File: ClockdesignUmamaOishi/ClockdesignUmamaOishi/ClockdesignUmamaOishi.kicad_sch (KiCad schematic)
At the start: 6 parts

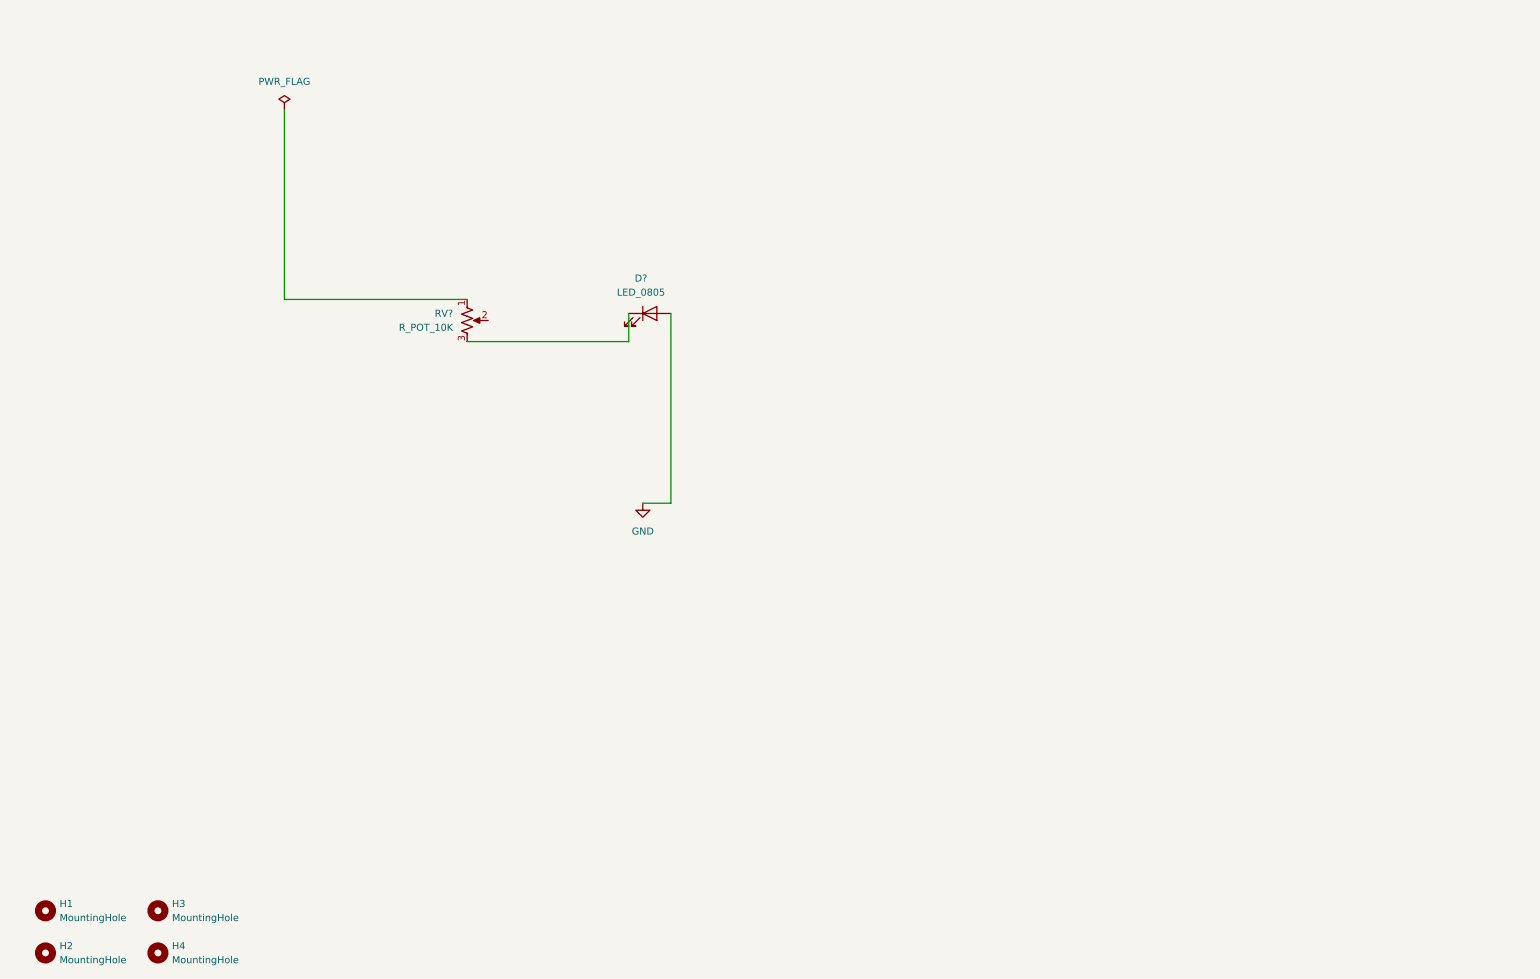
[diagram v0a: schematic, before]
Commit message: Week 2 schematics
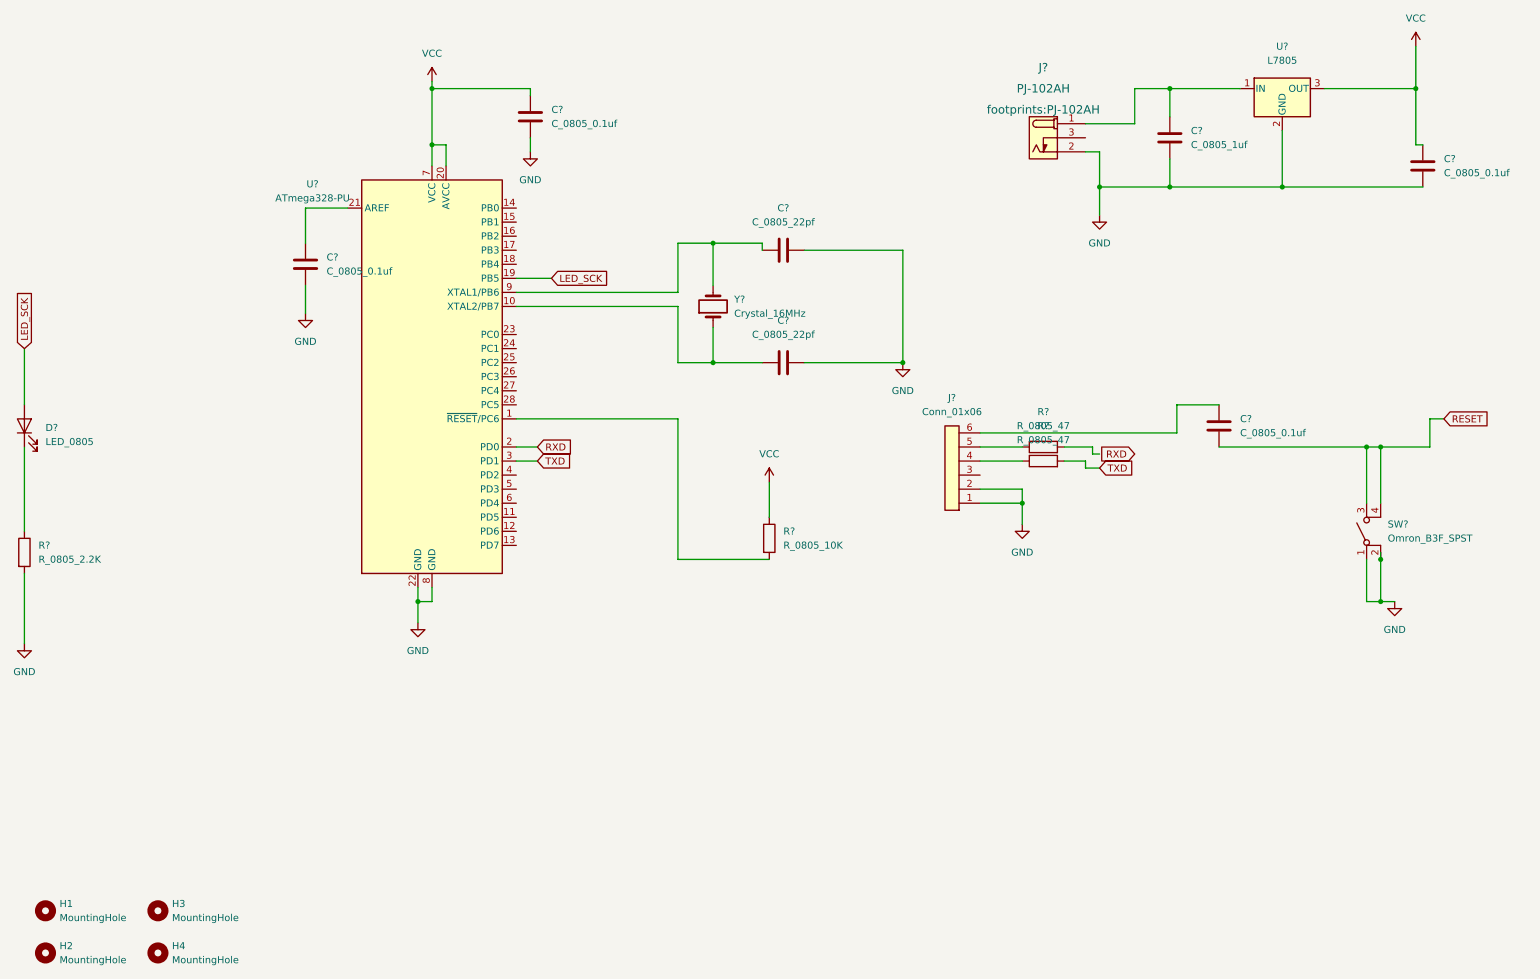
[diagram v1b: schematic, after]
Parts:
- removed D?: LED_0805, footprints:LED_0805_2012Metric, symbol HPS:LED_0805
- removed RV?: R_POT_10K, footprints:Potentiometer_Bourns_3386P_Vertical, symbol HPS:R_POT_10K
- added C? (x4): C_0805_0.1uf, footprints:C_0805_2012Metric, symbol HPS:C_0805_0.1uf
- added C?: C_0805_1uf, footprints:C_0805_2012Metric, symbol HPS:C_0805_1uf
- added C? (x2): C_0805_22pf, footprints:C_0805_2012Metric, symbol HPS:C_0805_22pf
- added D?: LED_0805, footprints:LED_0805_2012Metric, symbol HPS:LED_0805
- added J?: Conn_01x06, footprints:PinHeader_1x06_P2.54mm_Vertical, symbol HPS:Conn_01x06
- added J?: PJ-102AH, footprints:PJ-102AH, symbol HPS:PJ-102AH
- added R?: R_0805_10K, footprints:R_0805_2012Metric, symbol HPS:R_0805_10K
- added R?: R_0805_2.2K, footprints:R_0805_2012Metric, symbol HPS:R_0805_2.2K
- added R? (x2): R_0805_47, footprints:R_0805_2012Metric, symbol HPS:R_0805_47
- added SW?: Omron_B3F_SPST, footprints:SW_SPST_Omron_B3FS-100xP, symbol HPS:Omron_B3F_SPST
- added U?: L7805, symbol HPS:L7805
- added U?: ATmega328-PU, footprints:DIP-28_W7.62mm, symbol HPS:ATmega328-PU
- added Y?: Crystal_16MHz, footprints:Crystal_SMD_HC49-SD, symbol HPS:Crystal_16MHz
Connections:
- net GND: now also C?.2, C?.2, C?.2, C?.2, C?.2, C?.2, J?.1 (Pin_1), J?.2 (OUT), J?.2 (Pin_2), R?.2, SW?.1 (A), SW?.2 (A), U?.2 (GND), U?.22 (GND), U?.8 (GND)
- new net: C?.1, J?.1 (POLE), U?.1 (IN)
- new net: R?.2, U?.1 (~{RESET}/PC6)
- new net: J?.4 (Pin_4), R?.1
- new net: J?.5 (Pin_5), R?.1
- new net: C?.1, J?.6 (Pin_6)
- new net: C?.1, U?.9 (XTAL1/PB6), Y?.2
- new net: D?.1 (K), R?.1
- new net: C?.1, U?.21 (AREF)
- new net: C?.1, U?.10 (XTAL2/PB7), Y?.1
- new net LED_SCK: D?.2 (A), U?.19 (PB5)
- new net RESET: C?.2, SW?.3 (B), SW?.4 (B)
- new net RXD: U?.2 (PD0)
- new net TXD: R?.2, U?.3 (PD1)
- new net VCC: C?.1, C?.1, R?.1, U?.20 (AVCC), U?.3 (OUT), U?.7 (VCC)
